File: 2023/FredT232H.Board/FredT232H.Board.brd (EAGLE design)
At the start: 88 x 77 mm, 22 parts

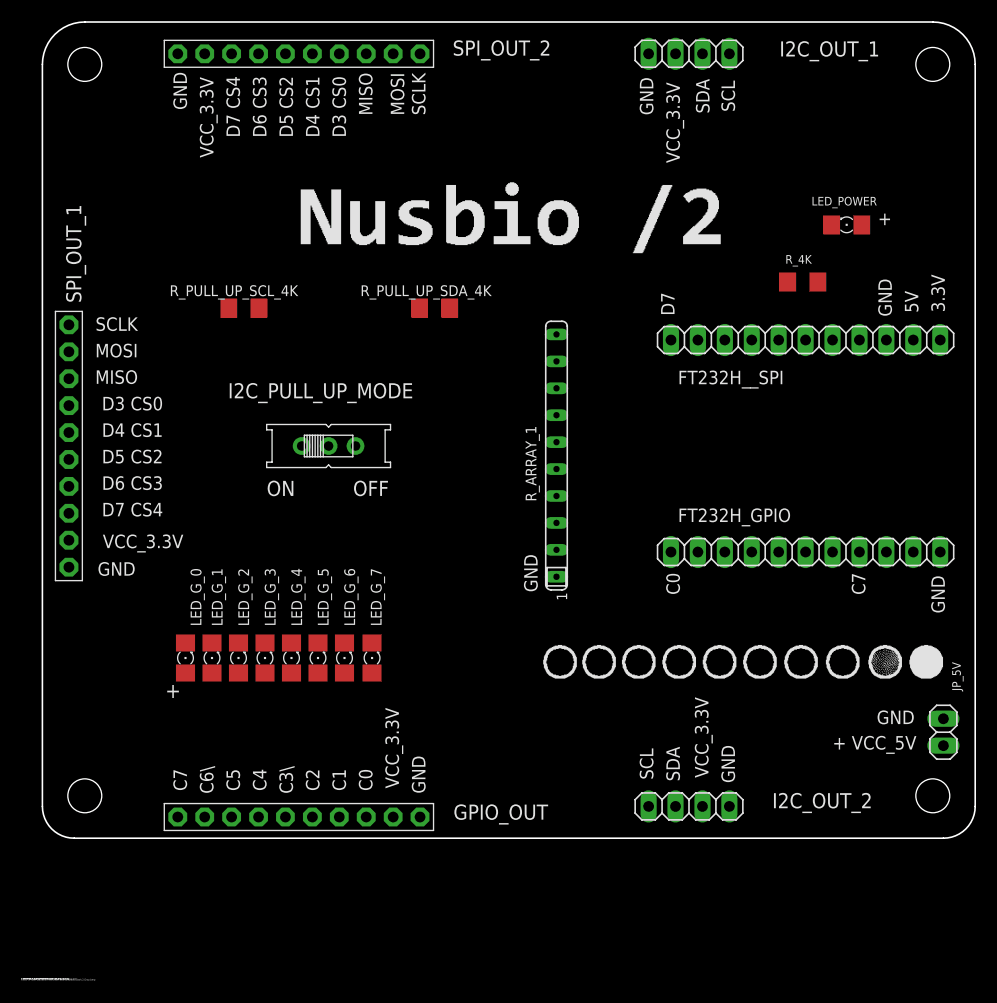
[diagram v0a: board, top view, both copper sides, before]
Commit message: More on FT232 board
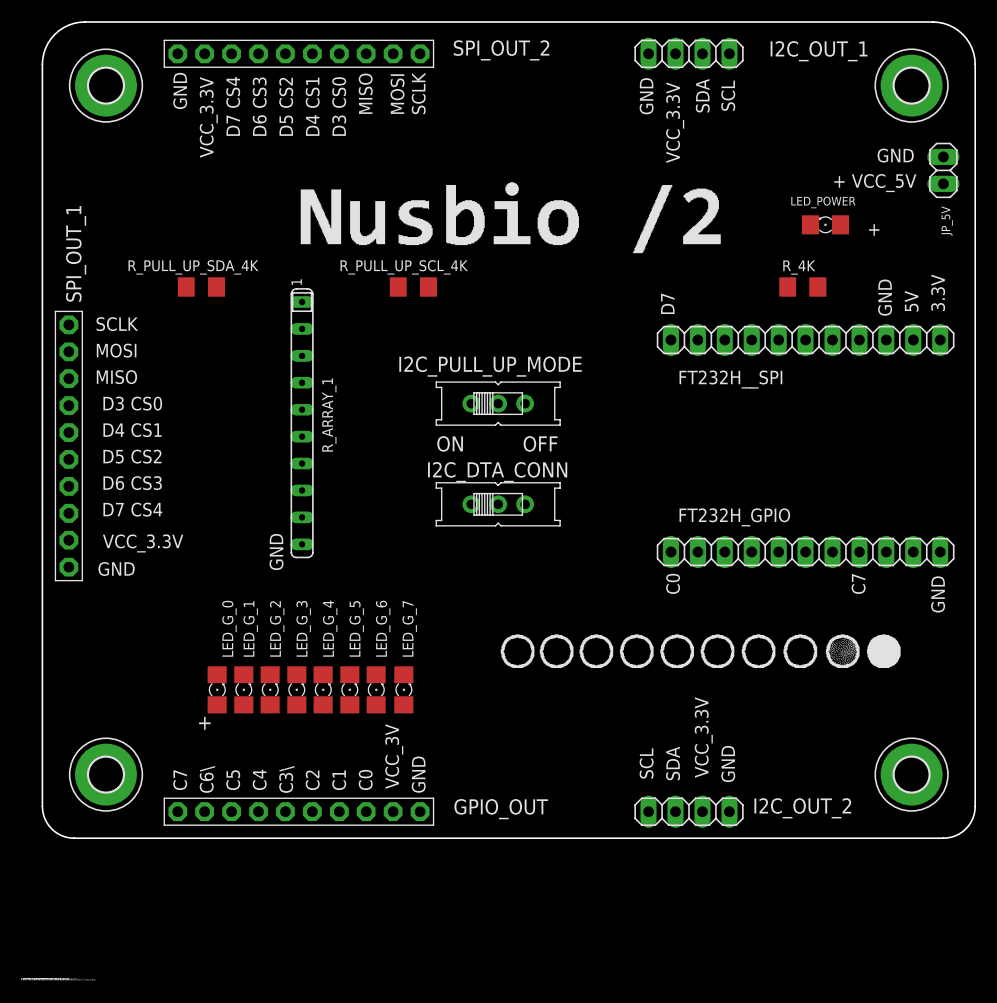
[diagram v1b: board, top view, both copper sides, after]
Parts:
- added H1, H2, H3, H4: MOUNT-PAD-ROUND3.3, holes:3,3-PAD
- added I2C_DTA_CONN: (no value), adafruit:EG1218
- moved JP_5V 53.0 mm to (87.0, 76.0)
- moved R_ARRAY_1 24.2 mm to (26.5, 52.1), turned to 270 degrees
- moved R_PULL_UP_SDA_4K 22.1 mm to (17.0, 65.0)
- moved I2C_PULL_UP_MODE 16.5 mm to (45.0, 54.0)
- moved R_PULL_UP_SCL_4K 16.1 mm to (37.0, 65.0)
- moved LED_G_0 4.24 mm to (18.5, 27.0)
- moved LED_G_1 4.24 mm to (21.0, 27.0)
- moved LED_G_2 4.24 mm to (23.5, 27.0)
- moved LED_G_3 4.24 mm to (26.0, 27.0)
- moved LED_G_4 4.24 mm to (28.5, 27.0)
- moved LED_G_5 4.24 mm to (31.0, 27.0)
- moved LED_G_6 4.24 mm to (33.5, 27.0)
- moved LED_G_7 4.24 mm to (36.1, 27.0)
- moved LED_POWER 2.00 mm to (75.9, 70.9)
- moved GPIO_OUT 0.50 mm to (26.2, 15.5)
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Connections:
- net D1_MOSI: now also I2C_DTA_CONN.P
- net D2_MISO: now also I2C_DTA_CONN.O
- net GND: now also H1.B3,3, H2.B3,3, H3.B3,3, H4.B3,3
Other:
- board text added: "VCC_3V"
